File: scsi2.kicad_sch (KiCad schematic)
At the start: 1 part, among them U4 NCR53c710 SCSI Host Controller

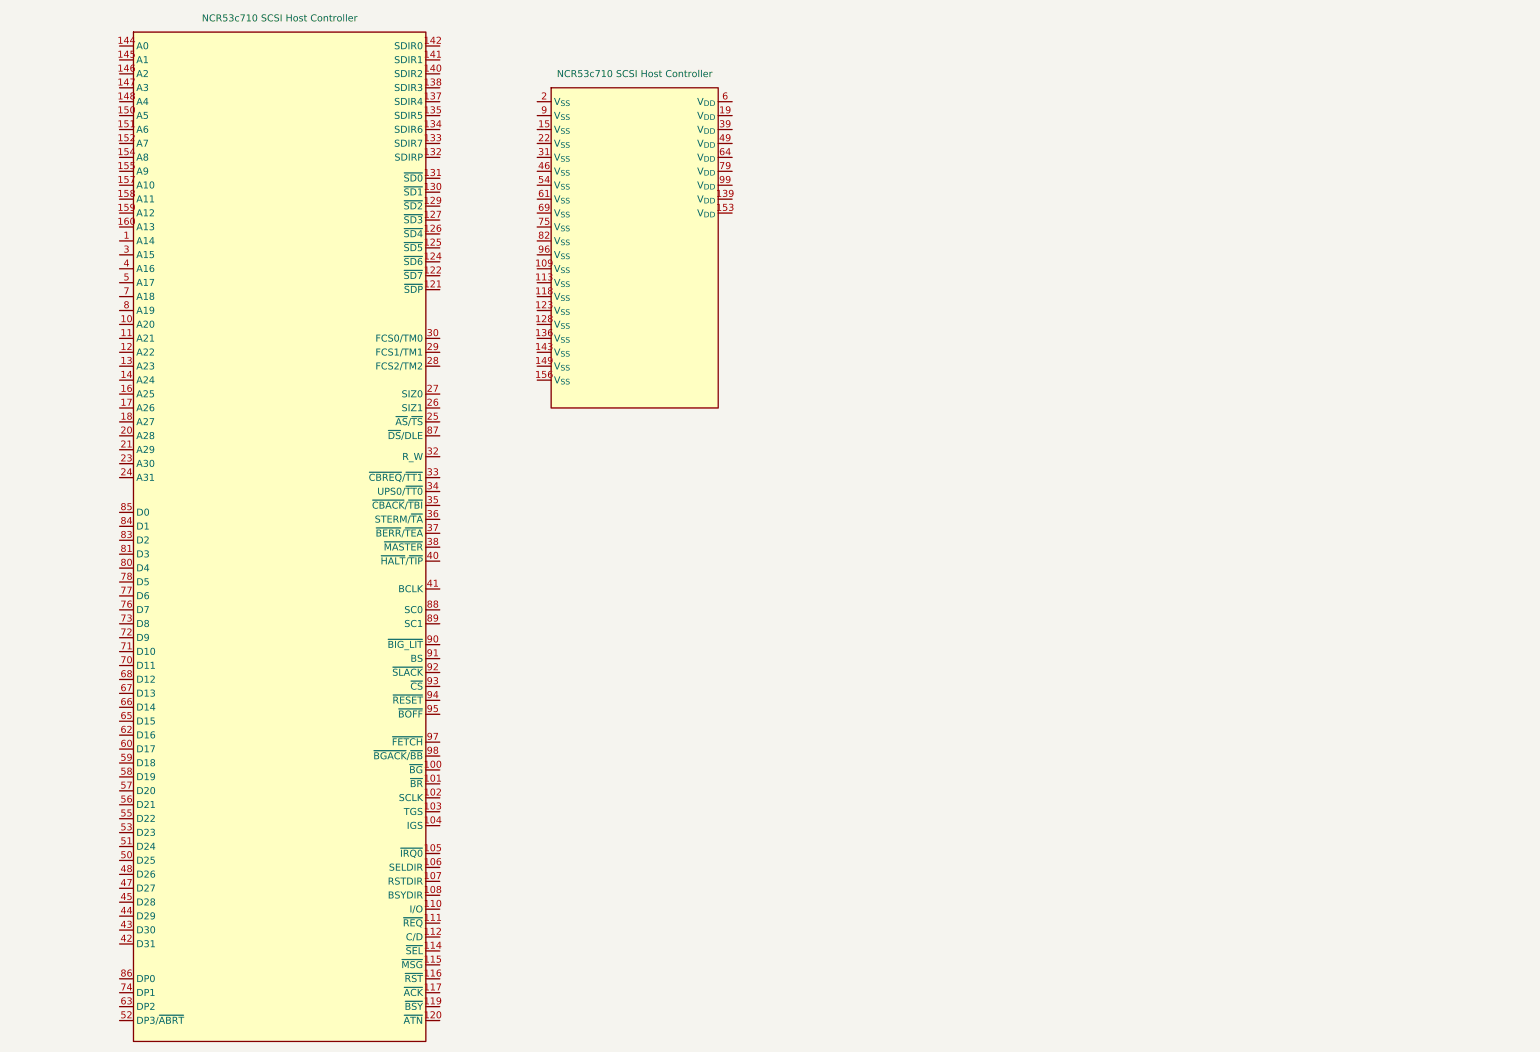
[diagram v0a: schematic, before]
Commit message: Update design
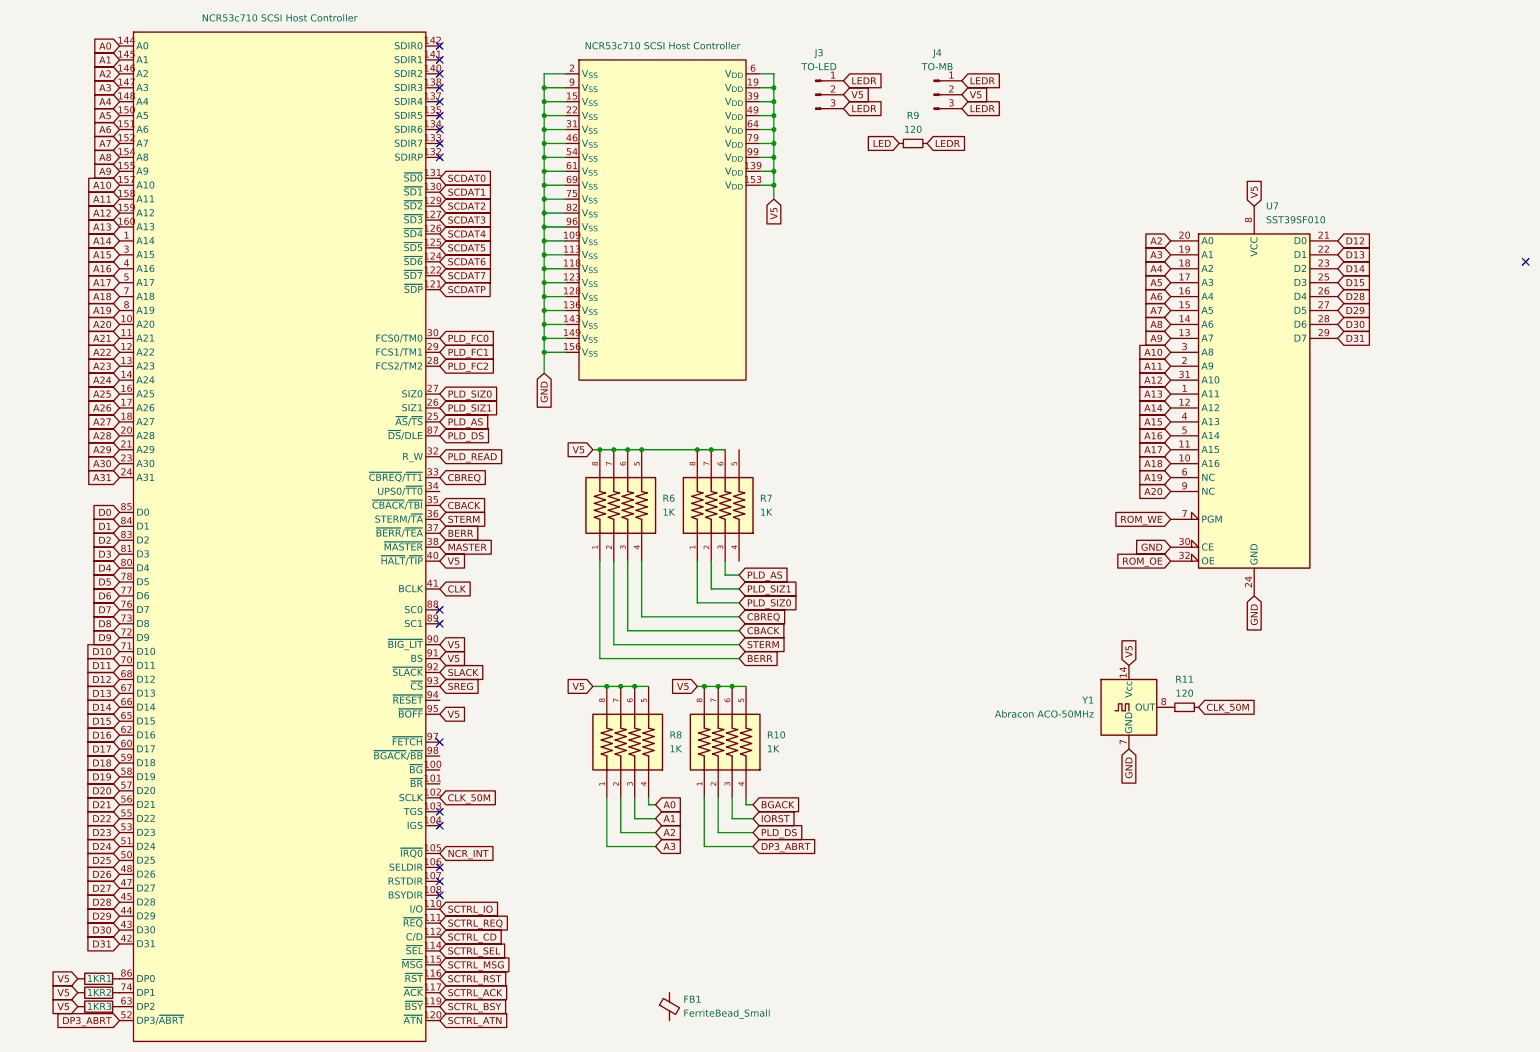
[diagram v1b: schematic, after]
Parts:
- added FB1: FerriteBead_Small, symbol Device:FerriteBead_Small
- added J3: TO-LED, Connector_PinHeader_2.54mm:PinHeader_1x03_P2.54mm_Vertical, symbol Connector:Conn_01x03_Pin
- added J4: TO-MB, Connector_PinHeader_2.54mm:PinHeader_1x03_P2.54mm_Vertical, symbol Connector:Conn_01x03_Pin
- added R1, R2, R3: 1K, symbol Device:R
- added R10, R6, R7, R8: 1K, YC324-FK-071KL:RESCAXS127P508X320X70-8N, symbol YC324-FK-071KL:YC324-FK-071KL
- added R11, R9: 120, Resistor_SMD:R_0603_1608Metric, symbol Device:R_Small
- added U7: SST39SF010, Package_SO:TSSOP-32_8x11mm_P0.65mm, symbol 39SF010-TSOP:SST39SF010
- added Y1: Abracon ACO-50MHz, Oscillator:Oscillator_DIP-14, symbol Oscillator:ACO-xxxMHz
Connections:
- net GND: now reaches U4.109 (V_{SS})
- net GND: now also U4.113 (V_{SS}), U4.118 (V_{SS}), U4.123 (V_{SS}), U4.128 (V_{SS}), U4.136 (V_{SS}), U4.143 (V_{SS}), U4.149 (V_{SS}), U4.15 (V_{SS}), U4.156 (V_{SS}), U4.2 (V_{SS}), U4.22 (V_{SS}), U4.31 (V_{SS}), U4.46 (V_{SS}), U4.54 (V_{SS}), U4.61 (V_{SS}), U4.69 (V_{SS}), U4.75 (V_{SS}), U4.82 (V_{SS}), U4.9 (V_{SS}), U4.96 (V_{SS}), U7.24 (GND), U7.30 (CE), Y1.7 (GND)
- net V5: now reaches U4.139 (V_{DD})
- net V5: now also U4.153 (V_{DD}), U4.19 (V_{DD}), U4.39 (V_{DD}), U4.40 (~{HALT}/~{TIP}), U4.49 (V_{DD}), U4.6 (V_{DD}), U4.64 (V_{DD}), U4.79 (V_{DD}), U4.90 (~{BIG_LIT}), U4.91 (BS), U4.95 (~{BOFF}), U4.99 (V_{DD}), J3.2 (Pin_2), J4.2 (Pin_2), R1.1, R10.5, R10.6, R10.7, R10.8, R2.1, R3.1, R6.5, R6.6, R6.7, R6.8, R7.6, R7.7, R7.8, R8.5, R8.6, R8.7, R8.8, U7.8 (VCC), Y1.14 (Vcc)
- net A14: now reaches U4.1 (A14)
- net A14: now also U7.12 (A12)
- net A20: now reaches U4.10 (A20)
- net A20: now also U7.9 (NC)
- net CLK_50M: now reaches U4.102 (SCLK)
- net CLK_50M: now also R11.2
- net NCR_INT: now reaches U4.105 (~{IRQ0})
- net A21: now reaches U4.11 (A21)
- net SCTRL_IO: now reaches U4.110 (I/O)
- net SCTRL_REQ: now reaches U4.111 (~{REQ})
- net SCTRL_CD: now reaches U4.112 (C/D)
- net SCTRL_SEL: now reaches U4.114 (~{SEL})
- net SCTRL_MSG: now reaches U4.115 (~{MSG})
- net SCTRL_RST: now reaches U4.116 (~{RST})
- net SCTRL_ACK: now reaches U4.117 (~{ACK})
- net SCTRL_BSY: now reaches U4.119 (~{BSY})
- net A22: now reaches U4.12 (A22)
- net SCTRL_ATN: now reaches U4.120 (~{ATN})
- net SCDATP: now reaches U4.121 (~{SDP})
- net SCDAT7: now reaches U4.122 (~{SD7})
- net SCDAT6: now reaches U4.124 (~{SD6})
- net SCDAT5: now reaches U4.125 (~{SD5})
- net SCDAT4: now reaches U4.126 (~{SD4})
- net SCDAT3: now reaches U4.127 (~{SD3})
- net SCDAT2: now reaches U4.129 (~{SD2})
- net A23: now reaches U4.13 (A23)
- net SCDAT1: now reaches U4.130 (~{SD1})
- net SCDAT0: now reaches U4.131 (~{SD0})
- net A24: now reaches U4.14 (A24)
- net A0: now reaches U4.144 (A0)
- net A0: now also R8.4
- net A1: now reaches U4.145 (A1)
- net A1: now also R8.3
- net A2: now reaches U4.146 (A2)
- net A2: now also R8.2, U7.20 (A0)
- net A3: now reaches U4.147 (A3)
- net A3: now also R8.1, U7.19 (A1)
- net A4: now reaches U4.148 (A4)
- net A4: now also U7.18 (A2)
- net A5: now reaches U4.150 (A5)
- net A5: now also U7.17 (A3)
- net A6: now reaches U4.151 (A6)
- net A6: now also U7.16 (A4)
- net A7: now reaches U4.152 (A7)
- net A7: now also U7.15 (A5)
- net A8: now reaches U4.154 (A8)
- net A8: now also U7.14 (A6)
- net A9: now reaches U4.155 (A9)
- net A9: now also U7.13 (A7)
- net A10: now reaches U4.157 (A10)
- net A10: now also U7.3 (A8)
- net A11: now reaches U4.158 (A11)
- net A11: now also U7.2 (A9)
- net A12: now reaches U4.159 (A12)
- net A12: now also U7.31 (A10)
- net A25: now reaches U4.16 (A25)
- net A13: now reaches U4.160 (A13)
- net A13: now also U7.1 (A11)
- net A26: now reaches U4.17 (A26)
- net A27: now reaches U4.18 (A27)
- net A28: now reaches U4.20 (A28)
- net A29: now reaches U4.21 (A29)
- net A30: now reaches U4.23 (A30)
- net A31: now reaches U4.24 (A31)
- net PLD_AS: now reaches U4.25 (~{AS}/~{TS})
- net PLD_AS: now also R7.3
- net PLD_SIZ1: now reaches U4.26 (SIZ1)
- net PLD_SIZ1: now also R7.2
- net PLD_SIZ0: now reaches U4.27 (SIZ0)
- net PLD_SIZ0: now also R7.1
- net PLD_FC2: now reaches U4.28 (FCS2/TM2)
- net PLD_FC1: now reaches U4.29 (FCS1/TM1)
- net A15: now reaches U4.3 (A15)
- net A15: now also U7.4 (A13)
- net PLD_FC0: now reaches U4.30 (FCS0/TM0)
- net PLD_READ: now reaches U4.32 (R_W)
- net CBREQ: now reaches U4.33 (~{CBREQ}/~{TT1})
- net CBREQ: now also R6.4
- net CBACK: now reaches U4.35 (~{CBACK}/~{TBI})
- net CBACK: now also R6.3
- net STERM: now reaches U4.36 (STERM/~{TA})
- net STERM: now also R6.2
- net BERR: now reaches U4.37 (~{BERR}/~{TEA})
- net BERR: now also R6.1
- net MASTER: now reaches U4.38 (~{MASTER})
- net A16: now reaches U4.4 (A16)
- net A16: now also U7.5 (A14)
- net CLK: now reaches U4.41 (BCLK)
- net D31: now reaches U4.42 (D31)
- net D31: now also U7.29 (D7)
- net D30: now reaches U4.43 (D30)
- net D30: now also U7.28 (D6)
- net D29: now reaches U4.44 (D29)
- net D29: now also U7.27 (D5)
- net D28: now reaches U4.45 (D28)
- net D28: now also U7.26 (D4)
- net D27: now reaches U4.47 (D27)
- net D26: now reaches U4.48 (D26)
- net A17: now reaches U4.5 (A17)
- net A17: now also U7.11 (A15)
- net D25: now reaches U4.50 (D25)
- net D24: now reaches U4.51 (D24)
- net DP3_ABRT: now reaches U4.52 (DP3/~{ABRT})
- net DP3_ABRT: now also R10.1
- net D23: now reaches U4.53 (D23)
- net D22: now reaches U4.55 (D22)
- net D21: now reaches U4.56 (D21)
- net D20: now reaches U4.57 (D20)
- net D19: now reaches U4.58 (D19)
- net D18: now reaches U4.59 (D18)
- net D17: now reaches U4.60 (D17)
- net D16: now reaches U4.62 (D16)
- net at U4.63 (DP2): now also R3.2
- net D15: now reaches U4.65 (D15)
- net D15: now also U7.25 (D3)
- net D14: now reaches U4.66 (D14)
- net D14: now also U7.23 (D2)
- net D13: now reaches U4.67 (D13)
- net D13: now also U7.22 (D1)
- net D12: now reaches U4.68 (D12)
- net D12: now also U7.21 (D0)
- net A18: now reaches U4.7 (A18)
- net A18: now also U7.10 (A16)
- net D11: now reaches U4.70 (D11)
- net D10: now reaches U4.71 (D10)
- net D9: now reaches U4.72 (D9)
- net D8: now reaches U4.73 (D8)
- net at U4.74 (DP1): now also R2.2
- net D7: now reaches U4.76 (D7)
- net D6: now reaches U4.77 (D6)
- net D5: now reaches U4.78 (D5)
- net A19: now reaches U4.8 (A19)
- net A19: now also U7.6 (NC)
- net D4: now reaches U4.80 (D4)
- net D3: now reaches U4.81 (D3)
- net D2: now reaches U4.83 (D2)
- net D1: now reaches U4.84 (D1)
- net D0: now reaches U4.85 (D0)
- net at U4.86 (DP0): now also R1.2
- net PLD_DS: now reaches U4.87 (~{DS}/DLE)
- net PLD_DS: now also R10.2
- net SLACK: now reaches U4.92 (~{SLACK})
- net SREG: now reaches U4.93 (~{CS})
- new net: R11.1, Y1.8 (OUT)
- new net BGACK: R10.4
- new net IORST: R10.3
- new net LED: R9.1
- new net LEDR: J3.1 (Pin_1), J3.3 (Pin_3), J4.1 (Pin_1), J4.3 (Pin_3), R9.2
- new net ROM_OE: U7.32 (OE)
- new net ROM_WE: U7.7 (PGM)
- no-connect marks 0 -> 18

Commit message: More work. Getting there.
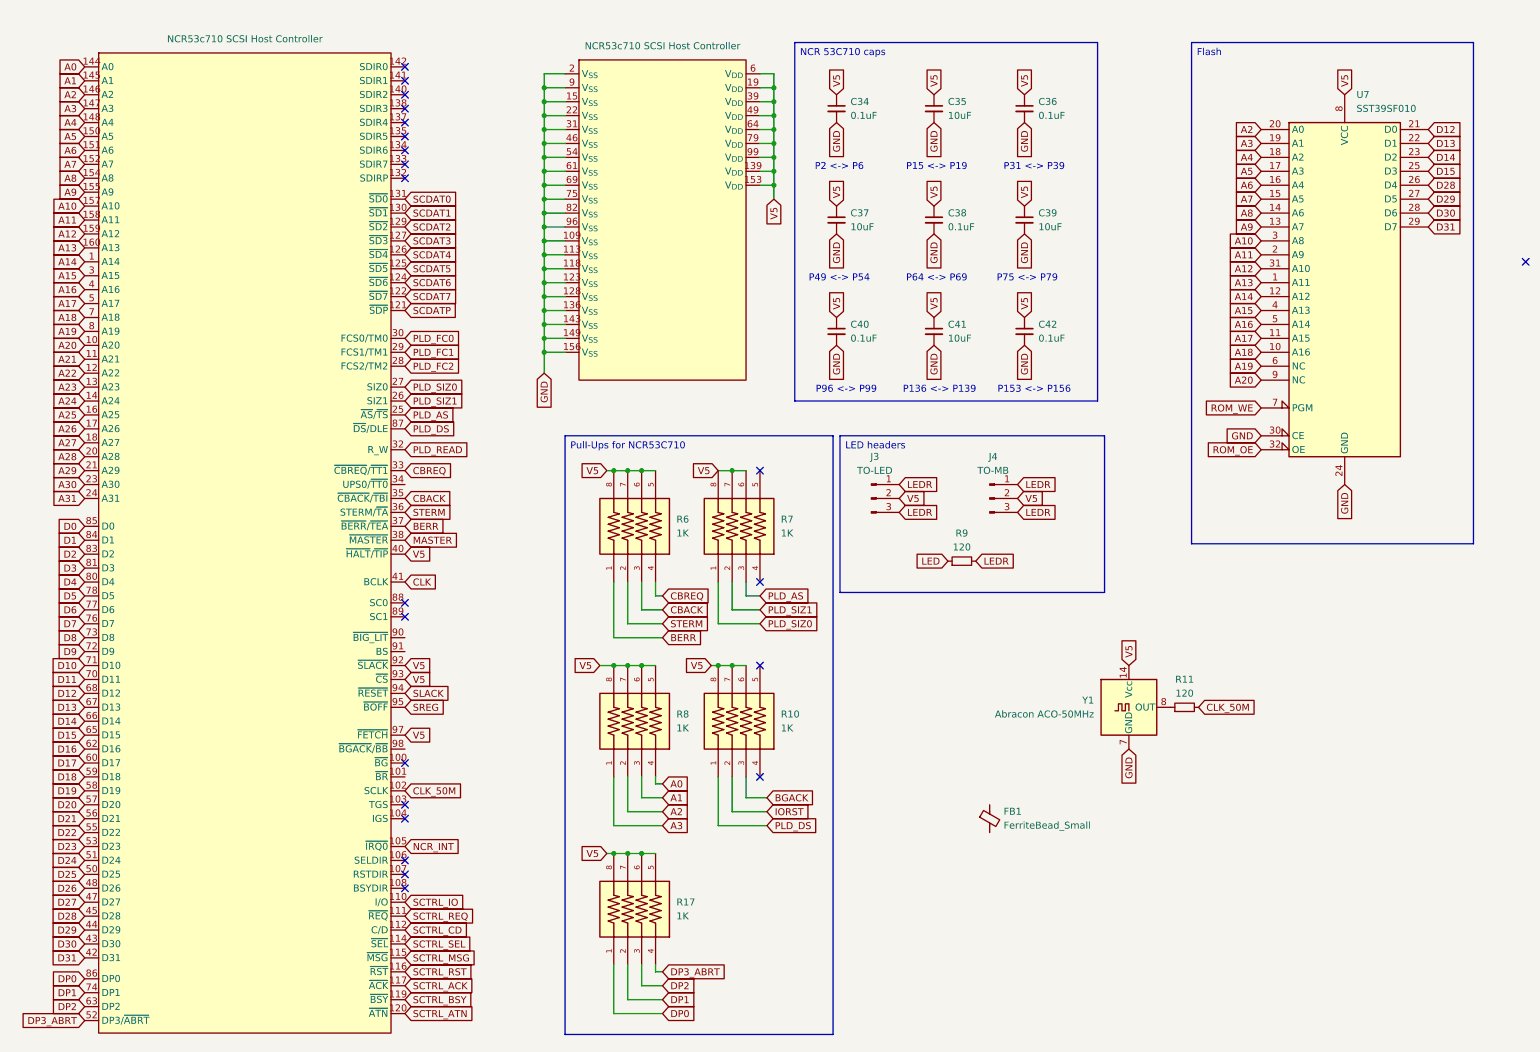
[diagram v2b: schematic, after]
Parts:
- removed R1, R2, R3: 1K, symbol Device:R
- added C34, C36, C38, C40, C42: 0.1uF, symbol Device:C_Small
- added C35, C37, C39, C41: 10uF, symbol Device:C_Small
- added R17: 1K, YC324-FK-071KL:RESCAXS127P508X320X70-8N, symbol YC324-FK-071KL:YC324-FK-071KL
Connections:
- net BGACK: now also R10.3; no longer R10.4
- net DP3_ABRT: now also R17.4; no longer R10.1
- net GND: now also C34.2, C35.2, C36.2, C37.2, C38.2, C39.2, C40.2, C41.2, C42.2
- net IORST: now also R10.2; no longer R10.3
- net PLD_DS: now also R10.1; no longer R10.2
- net SLACK: now also U4.94 (~{RESET}); no longer U4.92 (~{SLACK})
- net SREG: now also U4.95 (~{BOFF}); no longer U4.93 (~{CS})
- net V5: now also U4.92 (~{SLACK}), U4.93 (~{CS}), U4.97 (~{FETCH}), C34.1, C35.1, C36.1, C37.1, C38.1, C39.1, C40.1, C41.1, C42.1, R17.5, R17.6, R17.7, R17.8; no longer R10.5, U4.90 (~{BIG_LIT}), U4.91 (BS), U4.95 (~{BOFF})
- net DP1: now reaches U4.74 (DP1)
- net DP1: now also R17.2
- net DP0: now reaches U4.86 (DP0)
- net DP0: now also R17.1
- net DP2: now reaches U4.63 (DP2)
- net DP2: now also R17.3
- no-connect marks 18 -> 22
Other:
- note added: "P136 <-> P139"
- note added: "P15 <-> P19"
- note added: "P153 <-> P156"
- note added: "P2 <-> P6"
- note added: "P31 <-> P39"
- note added: "P49 <-> P54"
- note added: "P64 <-> P69"
- note added: "P75 <-> P79"
- note added: "P96 <-> P99"
- moved on the sheet: FB1, J3, J4, R10, R6, R7, R8, R9, U7
